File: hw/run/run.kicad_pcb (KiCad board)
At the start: 2 copper layers, 38.4 x 58.9 mm, 21 parts, among them J1 conn_trigger, J2 conn_done, J3 FTDI, J4 conn_active, SW1 switch_active, SW2 switch_active, SW3 switch_reset, U1 ATmega328P-PU, Y1 Crystal

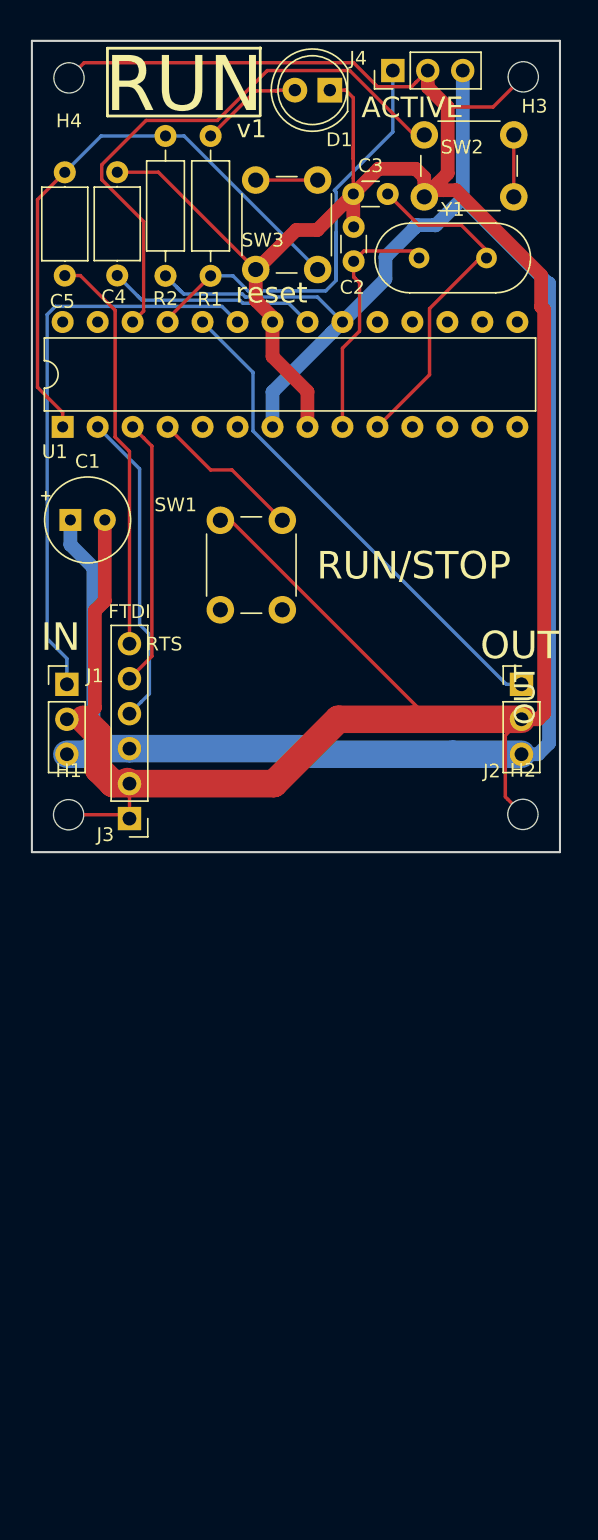
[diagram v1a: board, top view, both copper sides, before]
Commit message: RUN block v2
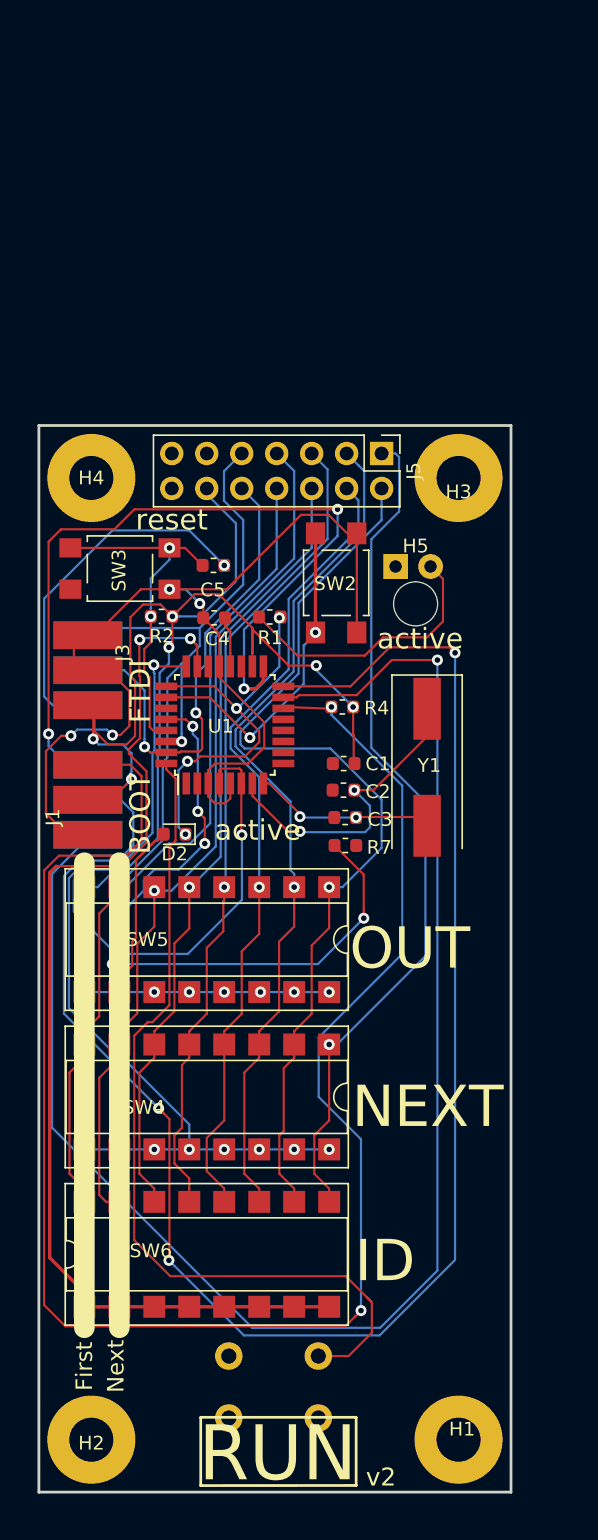
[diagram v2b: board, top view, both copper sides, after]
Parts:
- removed J2: conn_done, Connector_PinHeader_2.54mm:PinHeader_1x03_P2.54mm_Vertical
- removed J4: conn_active, Connector_PinHeader_2.54mm:PinHeader_1x03_P2.54mm_Vertical
- added D2: DIODE, Diode_SMD:D_0603_1608Metric, F.Cu at (134.1, 122.7)
- added H5: led_spy_hole, MountingHole:MountingHole_3.2mm_M3, F.Cu at (151.6, 105.9)
- added J5: BUS, Connector_PinHeader_2.54mm:PinHeader_2x07_P2.54mm_Vertical, F.Cu at (149.1, 95.0)
- added R4: 10k, Resistor_SMD:R_0603_1608Metric, F.Cu at (146.2, 113.4)
- added R7: 1k, Resistor_SMD:R_0603_1608Metric, F.Cu at (146.5, 123.5)
- added SW4: NEXT, Package_DIP:DIP-16_W7.62mm_SMDSocket_SmallPads, F.Cu at (136.4, 141.7)
- added SW5: ACTIVE, Package_DIP:DIP-16_W7.62mm_SMDSocket_SmallPads, F.Cu at (136.4, 130.3)
- added SW6: ID, Package_DIP:DIP-16_W7.62mm_SMDSocket_SmallPads, F.Cu at (136.4, 153.2)
- C1: footprint Capacitor_THT:CP_Radial_Tantal_D6.0mm_P2.50mm -> Capacitor_SMD:C_0603_1608Metric
- C2, C3: footprint Capacitor_THT:C_Disc_D3.0mm_W1.6mm_P2.50mm -> Capacitor_SMD:C_0603_1608Metric
- C4, C5: footprint Capacitor_THT:C_Axial_L5.1mm_D3.1mm_P7.50mm_Horizontal -> Capacitor_SMD:C_0603_1608Metric
- D1: moved to B.Cu
- H1, H2, H3, H4: footprint MountingHole:MountingHole_2.2mm_M2 -> MountingHole:MountingHole_3.2mm_M3_Pad
- J1: value conn_trigger -> bootloader; footprint Connector_PinHeader_2.54mm:PinHeader_1x03_P2.54mm_Vertical -> autoblocks:edge_connector_3
- J3: footprint Connector_PinHeader_2.54mm:PinHeader_1x06_P2.54mm_Vertical -> autoblocks:edge_connector_3
- R1, R2: footprint Resistor_THT:R_Axial_DIN0207_L6.3mm_D2.5mm_P10.16mm_Horizontal -> Resistor_SMD:R_0603_1608Metric
- SW1: value switch_active -> runSwitch; moved to B.Cu
- SW2: value switch_active -> active; footprint autoblocks:SW_PUSH_6mm_H5mm -> Button_Switch_SMD:SW_SPST_TL3305C
- SW3: value switch_reset -> reset; footprint autoblocks:SW_PUSH_6mm_H5mm -> Button_Switch_SMD:SW_SPST_TL3305C
- U1: value ATmega328P-PU -> ATmega328-AU; footprint Package_DIP:DIP-28_W7.62mm -> Package_QFP:TQFP-32_7x7mm_P0.8mm
- Y1: footprint Crystal:Crystal_HC18-U_Vertical -> Crystal:Crystal_SMD_HC49-SD
- moved SW1 60.8 mm to (144.5, 160.6), turned to 180 degrees
- moved H2 55.2 mm to (128.0, 166.6)
- moved H1 53.5 mm to (154.7, 166.6)
- moved C3 45.3 mm to (146.5, 121.4)
- moved C2 40.9 mm to (146.3, 119.4), turned to 0 degrees
- moved Y1 37.0 mm to (152.4, 117.8), turned to 270 degrees
- moved R1 35.2 mm to (141.0, 106.9), turned to 0 degrees
- moved D1 34.9 mm to (150.1, 103.2), turned to 0 degrees
- moved SW2 33.2 mm to (145.8, 104.4), turned to 90 degrees
- moved C5 30.5 mm to (136.9, 103.1), turned to 0 degrees
- moved H3 29.5 mm to (154.7, 96.8)
- moved H4 29.1 mm to (128.0, 96.8)
- moved C1 26.6 mm to (146.3, 117.5), turned to 180 degrees
- moved C4 25.8 mm to (136.9, 106.9), turned to 180 degrees
- moved R2 24.7 mm to (133.1, 106.8), turned to 180 degrees
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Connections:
- C1 pad 1: VCC -> bus11
- C1 pad 2: GND -> bus13
- C2 pad 1: GND -> bus13
- C3 pad 1: GND -> bus13
- C4 pad 2: GND -> bus13
- D1 pad 1: GND -> bus13
- H1 pad 1: GND -> Net-(H1-Pad1)
- H2 pad 1: GND -> Net-(H2-Pad1)
- H3 pad 1: GND -> Net-(H3-Pad1)
- H4 pad 1: GND -> Net-(H4-Pad1)
- J1 pad 1: a0 -> bus13
- J1 pad 2: GND -> bus11
- J1 pad 3: VCC -> d10
- J3 pad 1: GND -> bus13
- J3 pad 2: GND -> bus13
- J3 pad 3: VCC -> bus11
- R2 pad 1: VCC -> bus11
- SW1 pad 2: GND -> bus13
- SW1 pad 3: Net-(SW1-Pad3) -> (no net)
- SW1 pad 4: Net-(SW1-Pad4) -> (no net)
- SW2 pad 2: GND -> bus13
- SW3 pad 1: GND -> bus13
- U1 pad 1: RESET -> d3
- U1 pad 10: XTAL2 -> d6
- U1 pad 11: d5 -> d7
- U1 pad 12: d6 -> d8
- U1 pad 13: d7 -> d9
- U1 pad 14: d8 -> d10
- U1 pad 15: d9 -> d11
- U1 pad 16: d10 -> d12
- U1 pad 17: d11 -> d13
- U1 pad 18: d12 -> bus11
- U1 pad 19: d13 -> Net-(U1-Pad19)
- U1 pad 2: RX -> d4
- U1 pad 20: VCC -> AREF
- U1 pad 21: AREF -> bus13
- U1 pad 22: GND -> Net-(U1-Pad22)
- U1 pad 3: TX -> bus13
- U1 pad 4: d2 -> bus11
- U1 pad 5: d3 -> bus13
- U1 pad 6: d4 -> bus11
- U1 pad 7: VCC -> XTAL1
- U1 pad 8: GND -> XTAL2
- U1 pad 9: XTAL1 -> d5
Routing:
- net GND: track 233.7 -> 0.00 mm
- net VCC: track 142.5 -> 0.00 mm
- net d10: track 0.00 -> 128.6 mm, vias 0 -> 2
- net d12: track 0.00 -> 126.1 mm, vias 0 -> 3
- net bus11: track 0.00 -> 125.6 mm, vias 0 -> 7
- net d11: track 0.00 -> 114.8 mm, vias 0 -> 1
- net bus13: track 0.00 -> 81.1 mm, vias 0 -> 4
- net bus2: track 0.00 -> 68.0 mm, vias 0 -> 1
- net bus7: track 0.00 -> 62.9 mm, vias 0 -> 1
- net bus3: track 0.00 -> 62.5 mm, vias 0 -> 1
- net bus1: track 0.00 -> 62.1 mm, vias 0 -> 1
- net bus5: track 0.00 -> 59.9 mm, vias 0 -> 1
- net bus8: track 0.00 -> 59.4 mm, vias 0 -> 1
- net bus4: track 0.00 -> 59.0 mm, vias 0 -> 1
- net d13: track 0.00 -> 58.8 mm, vias 0 -> 3
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- added copper zone on B.Cu, net bus11
- added copper zone on F.Cu, net bus13
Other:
- board size 38.4 x 58.9 mm -> 34.3 x 77.5 mm
- rule trace_min: 0.2 -> 0.16
- board text added: "BOOT"
- board text added: "FTDI"
- board text added: "First"
- board text added: "ID"
- board text added: "NEXT"
- board text added: "Next"
- board text added: "active"
- board text added: "v2"
- board text removed: "ACTIVE"
- board text removed: "IN"
- board text removed: "RTS"
- board text removed: "v1"
